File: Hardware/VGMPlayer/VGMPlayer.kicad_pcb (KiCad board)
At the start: 2 copper layers, 100 x 98.8 mm, 96 parts, among them J1 USB_B_Mini, J2 SD_Card, J3 LCD_PORT, Q1 9013, Q2 S8550, SW1 Mode, SW2 NEXT, SW3 PREV, SW4 SELECT, SW5 PWR, U1 STM32F103XX, U10 LTC6903, U11 HC-06, U12 R_POT_SW, U13 YM3012, U14 LM324, U19 ESP8266Module, U2 SDCardModule, U3 LM386, U4 LM386, U5 YM2151, U6 AUDIOJACK-VGM, U7 YM2612, U8 SN76489, U9 LTC6903

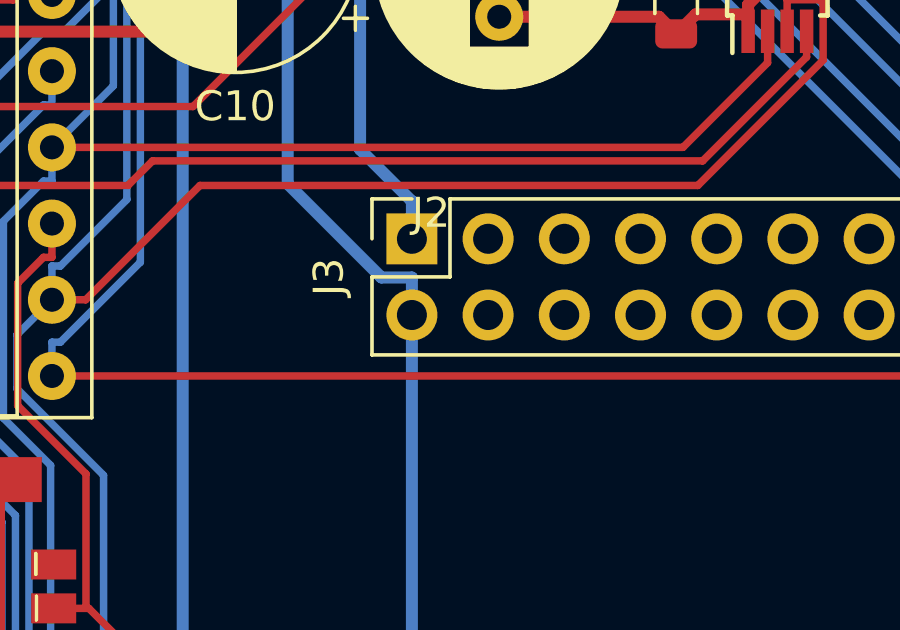
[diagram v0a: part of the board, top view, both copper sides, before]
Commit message: 1
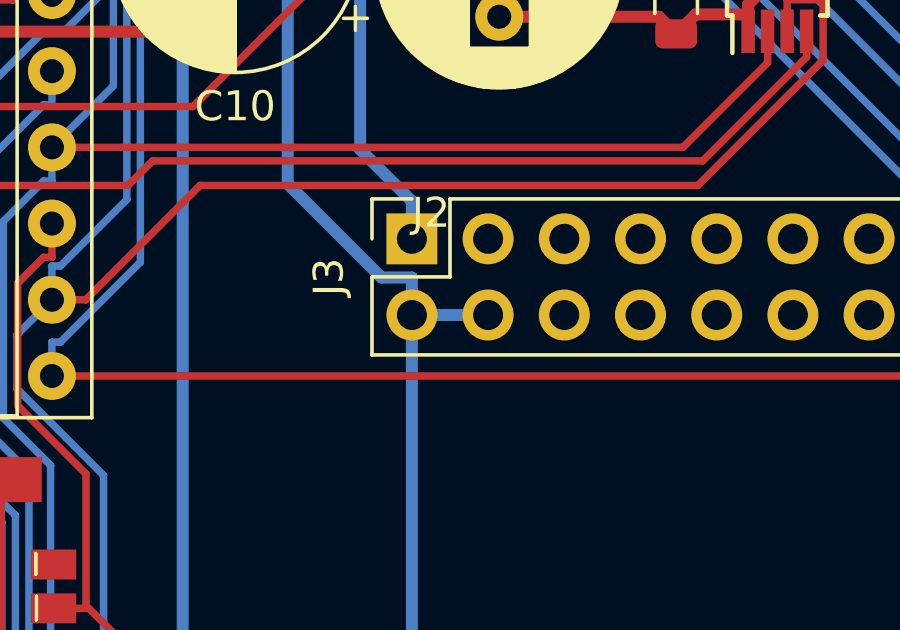
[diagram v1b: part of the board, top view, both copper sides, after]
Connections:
- J3 pad 4: Net-(J3-Pad4) -> +3V3
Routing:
- net +3V3: track 148.4 -> 150.9 mm

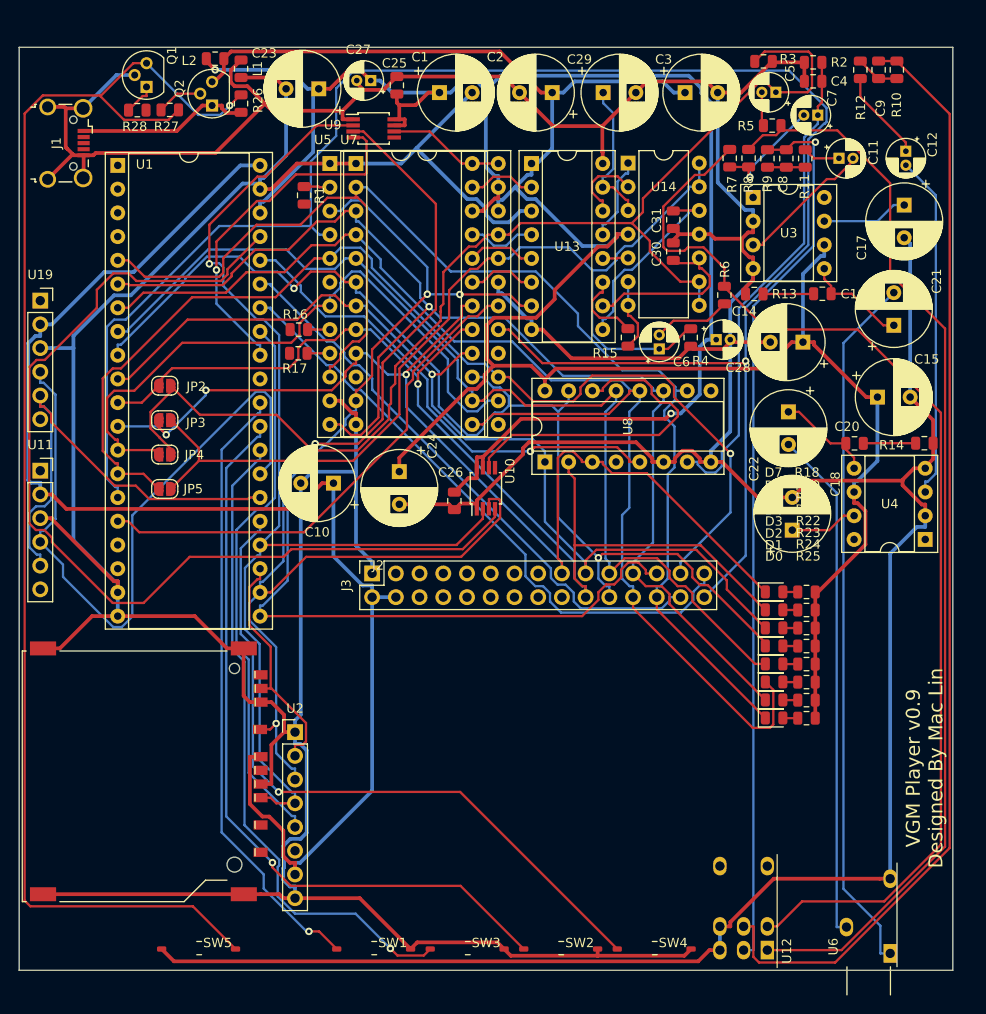
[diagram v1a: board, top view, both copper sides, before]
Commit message: 1
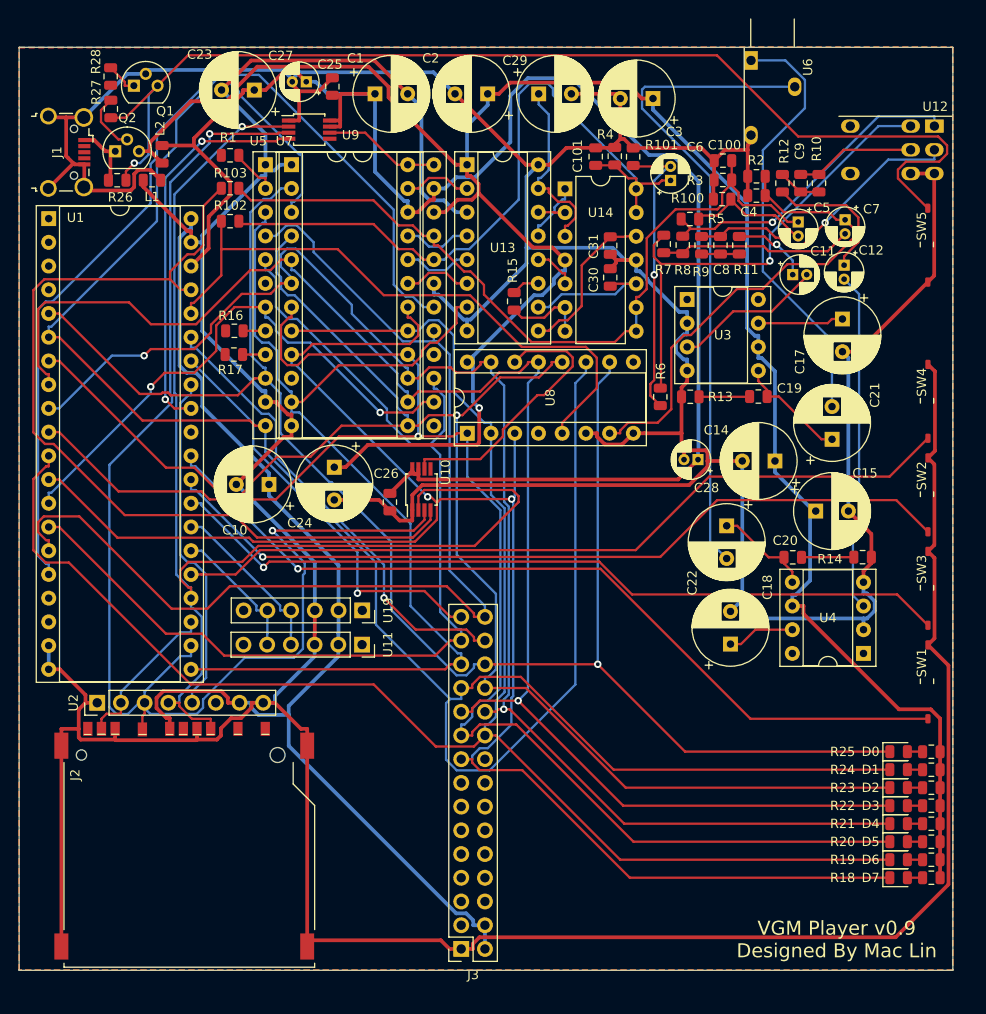
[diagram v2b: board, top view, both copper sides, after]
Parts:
- removed JP2, JP3, JP4, JP5: Jumper_NC_Small, Jumper:SolderJumper-2_P1.3mm_Open_RoundedPad1.0x1.5mm
- added C100: TBD, Capacitor_SMD:C_0805_2012Metric, F.Cu at (95.4, 34.5)
- added C101: TBD, Capacitor_SMD:C_0805_2012Metric, F.Cu at (81.7, 34.1)
- added R100: TBD, Resistor_SMD:R_0805_2012Metric, F.Cu at (95.3, 38.6)
- added R101: TBD, Resistor_SMD:R_0805_2012Metric, F.Cu at (85.8, 34.1)
- added R102: TBD, Resistor_SMD:R_0805_2012Metric, F.Cu at (42.6, 41.0)
- added R103: TBD, Resistor_SMD:R_0805_2012Metric, F.Cu at (42.6, 37.4)
- moved SW5 108.5 mm to (117.3, 43.5), turned to 90 degrees
- moved U12 90.0 mm to (118.0, 30.8), turned to 270 degrees
- moved U6 88.2 mm to (100.6, 27.8), turned to 0 degrees
- moved SW1 65.8 mm to (117.3, 90.3), turned to 90 degrees
- moved SW4 65.5 mm to (117.3, 60.2), turned to 90 degrees
- moved SW3 62.6 mm to (117.3, 80.3), turned to 90 degrees
- moved SW2 62.5 mm to (117.3, 70.2), turned to 90 degrees
- moved U19 47.8 mm to (56.8, 82.6), turned to 270 degrees
- moved J3 41.3 mm to (67.4, 118.9), turned to 180 degrees
- moved U11 39.2 mm to (56.7, 86.3), turned to 270 degrees
- moved R18 33.4 mm to (117.7, 111.3)
- moved D7 33.4 mm to (114.2, 111.3)
- moved R19 29.9 mm to (117.7, 109.3)
- moved D6 29.9 mm to (114.2, 109.3)
- moved R20 26.5 mm to (117.7, 107.4)
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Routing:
- net Net-(C9-Pad1): track 119.2 -> 12.9 mm
- net D1: track 133.6 -> 232.0 mm, vias 1 -> 0
- net A0: track 204.4 -> 115.8 mm, vias 1 -> 0
- net Net-(R5-Pad1): track 116.0 -> 34.8 mm, vias 0 -> 1
- net GNDA: track 442.4 -> 362.3 mm
- net Net-(R6-Pad1): track 121.0 -> 51.7 mm, vias 0 -> 1
- net D7: track 119.7 -> 186.2 mm, vias 3 -> 2
- net D6: track 117.3 -> 182.5 mm, vias 1 -> 0
- net Net-(C8-Pad1): track 95.8 -> 30.8 mm
- net D5: track 103.7 -> 168.5 mm
- net RXD: track 74.9 -> 18.4 mm
- net D3: track 111.6 -> 165.0 mm, vias 0 -> 1
- net A1: track 54.5 -> 100.8 mm
- net YM_MOL: track 127.2 -> 85.7 mm
- net D2: track 136.4 -> 173.9 mm, vias 0 -> 1
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- added copper zone on F.Cu, net (none)
- added copper zone on B.Cu, net GND
- added copper zone on F.Cu, net GND
